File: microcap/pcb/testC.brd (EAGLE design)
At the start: 100 parts

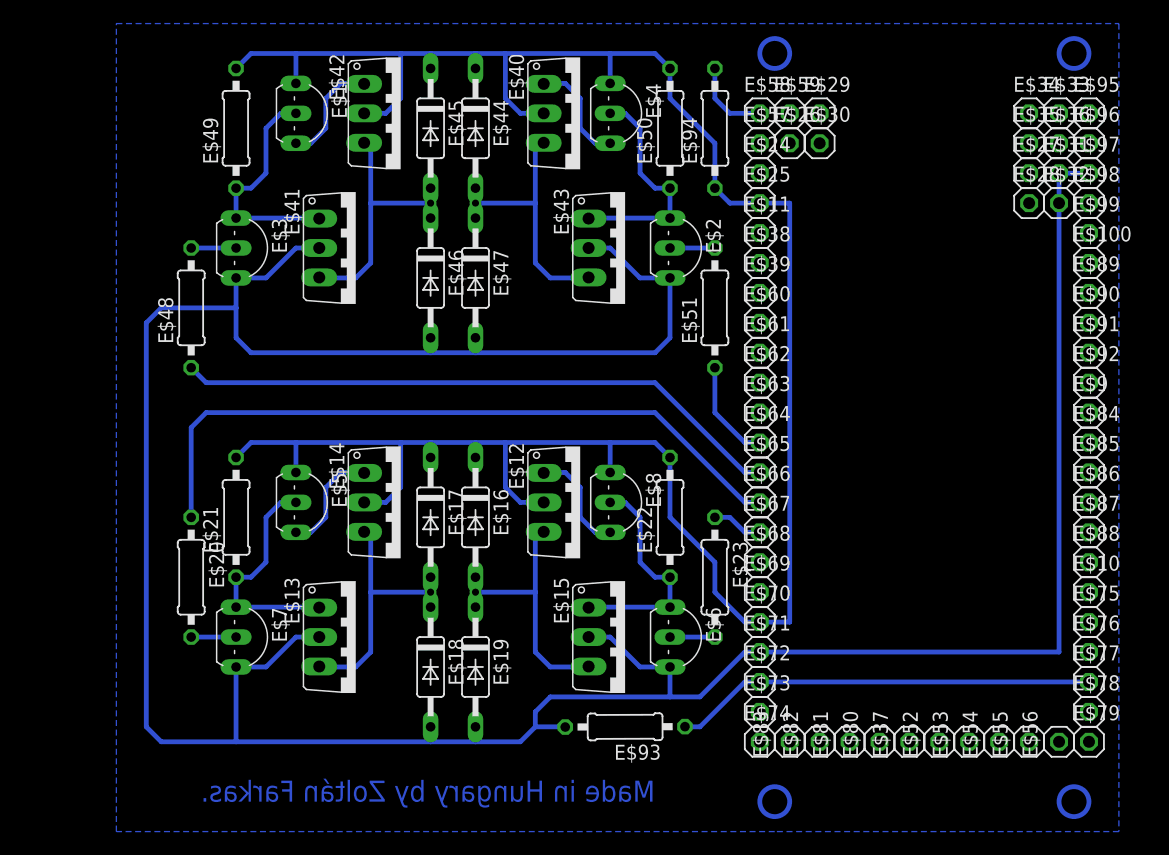
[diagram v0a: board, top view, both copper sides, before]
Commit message: pcb test update
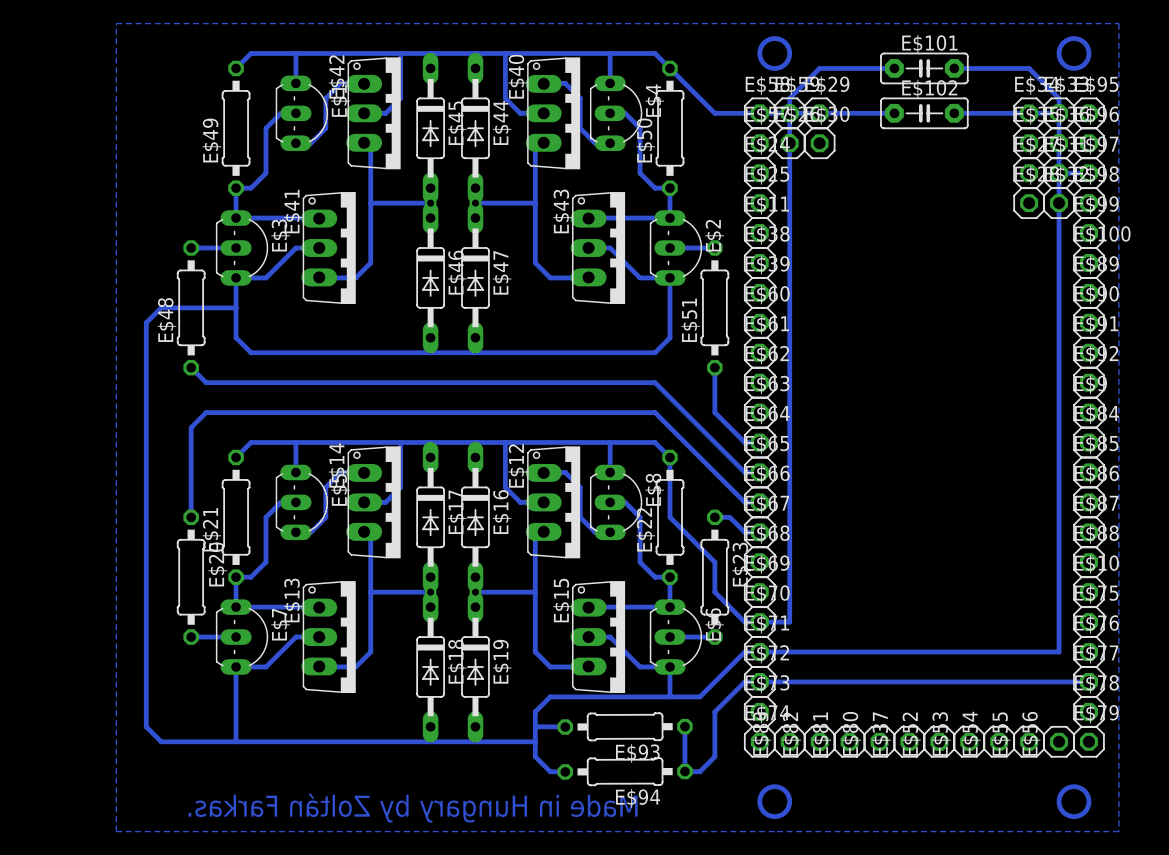
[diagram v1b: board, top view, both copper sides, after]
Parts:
- added E$101, E$102: (no value), capacitor-wima:C5B2.5
- moved E$94 55.1 mm to (71.1, 36.8), turned to 180.2 degrees
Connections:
- removed net S$29: E$1.C, E$16.C, E$17.C, E$21.2, E$22.2, E$25.1, E$4.C, E$44.C, E$45.C, E$49.2, E$5.C, E$50.2, E$70.1, E$8.C, E$94.1
- removed net S$30: E$58.1, E$94.2
- new net S$18: E$101.2, E$102.2, E$18.A, E$19.A, E$2.E, E$3.E, E$46.A, E$47.A, E$6.E, E$7.E, E$71.1, E$97.1
- net S$8: now also E$1.C, E$101.1, E$102.1, E$16.C, E$17.C, E$21.2, E$22.2, E$4.C, E$44.C, E$45.C, E$49.2, E$5.C, E$50.2, E$58.1, E$59.1, E$70.1, E$8.C; no longer E$18.A, E$19.A, E$2.E, E$3.E, E$46.A, E$47.A, E$6.E, E$7.E, E$71.1, E$97.1
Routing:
- net S$18: track 0.00 -> 291.9 mm
- net S$29: track 193.1 -> 0.00 mm
- net S$8: track 261.7 -> 213.9 mm
- net S$26: track 35.9 -> 43.5 mm
- net S$30: track 6.88 -> 0.00 mm
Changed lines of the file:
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@@
 <layer number="21" name="tPlace" color="7" fill="1" visible="yes" active="yes"/>
 <layer number="22" name="bPlace" color="7" fill="1" visible="yes" active="yes"/>
-<layer number="23" name="tOrigins" color="15" fill="1" visible="no" active="yes"/>
-<layer number="24" name="bOrigins" color="15" fill="1" visible="no" active="yes"/>
+<layer number="23" name="tOrigins" color="15" fill="1" visible="yes" active="yes"/>
+<layer number="24" name="bOrigins" color="15" fill="1" visible="yes" active="yes"/>
 <layer number="25" name="tNames" color="7" fill="1" visible="no" active="yes"/>
 <layer number="26" name="bNames" color="7" fill="1" visible="no" active="yes"/>
@@
 <circle x="109.22" y="34.29" radius="1.27" width="0.4064" layer="16"/>
 <circle x="83.82" y="34.29" radius="1.27" width="0.4064" layer="16"/>
-<text x="73.66" y="34.29" size="1.778" layer="16" rot="MR0">Made in Hungary by Zoltán Farkas.</text>
+<text x="72.39" y="33.02" size="1.778" layer="16" rot="MR0">Made in Hungary by Zoltán Farkas.</text>
 </plain>
 <attributes>
@@
 <element name="E$100" library="pinhead" package="1X01" value="" x="110.49" y="80.01"/>
 <element name="E$93" library="resistor" package="0207/10" value="" x="71.12" y="40.64" rot="R180.2"/>
-<element name="E$94" library="resistor" package="0207/10" value="" x="78.74" y="91.44" rot="R90"/>
+<element name="E$94" library="resistor" package="0207/10" value="" x="71.12" y="36.83" rot="R180.2"/>
+<element name="E$101" library="capacitor-wima" package="C5B2.5" value="" x="96.52" y="96.52"/>
+<element name="E$102" library="capacitor-wima" package="C5B2.5" value="" x="96.52" y="92.71"/>
 </elements>
 <signals>
@@
 <wire x1="74.93" y1="81.28" x2="78.74" y2="81.28" width="0.4064" layer="16"/>
 </signal>
-<signal name="S$8">
+<signal name="S$18">
+<wire x1="66.04" y1="36.83" x2="64.77" y2="36.83" width="0.4064" layer="16"/>
 <wire x1="69.85" y1="81.28" x2="68.58" y2="81.28" width="0.4064" layer="16"/>
 <wire x1="72.39" y1="78.74" x2="69.85" y2="81.28" width="0.4064" layer="16"/>
@@
 <wire x1="74.93" y1="45.72" x2="74.93" y2="43.18" width="0.4064" layer="16"/>
 <contactref element="E$18" pad="A"/>
-<wire x1="58.42" y1="39.37" x2="62.23" y2="39.37" width="0.4064" layer="16"/>
+<wire x1="58.42" y1="39.37" x2="63.5" y2="39.37" width="0.4064" layer="16"/>
 <wire x1="58.42" y1="40.64" x2="58.42" y2="39.37" width="0.4064" layer="16"/>
 <contactref element="E$7" pad="E"/>
@@
 <wire x1="63.5" y1="41.91" x2="63.5" y2="40.64" width="0.4064" layer="16"/>
 <wire x1="66.04" y1="40.64" x2="63.5" y2="40.64" width="0.4064" layer="16"/>
-<wire x1="63.5" y1="40.64" x2="62.23" y2="39.37" width="0.4064" layer="16"/>
+<wire x1="63.5" y1="38.1" x2="63.5" y2="39.37" width="0.4064" layer="16"/>
+<wire x1="63.5" y1="39.37" x2="63.5" y2="40.64" width="0.4064" layer="16"/>
+<wire x1="64.77" y1="36.83" x2="63.5" y2="38.1" width="0.4064" layer="16"/>
+<wire x1="107.95" y1="87.63" x2="107.95" y2="92.71" width="0.4064" layer="16"/>
+<contactref element="E$101" pad="2"/>
+<wire x1="107.95" y1="92.71" x2="107.95" y2="93.98" width="0.4064" layer="16"/>
+<wire x1="99.06" y1="96.52" x2="105.41" y2="96.52" width="0.4064" layer="16"/>
+<wire x1="105.41" y1="96.52" x2="107.95" y2="93.98" width="0.4064" layer="16"/>
+<contactref element="E$102" pad="2"/>
+<wire x1="99.06" y1="92.71" x2="107.95" y2="92.71" width="0.4064" layer="16"/>
 </signal>
 <signal name="S$1">
@@
 </signal>
 <signal name="S$26">
+<wire x1="76.2" y1="36.83" x2="77.47" y2="36.83" width="0.4064" layer="16"/>
+<wire x1="77.47" y1="36.83" x2="78.74" y2="38.1" width="0.4064" layer="16"/>
 <contactref element="E$77" pad="1"/>
 <wire x1="110.49" y1="44.45" x2="81.28" y2="44.45" width="0.4064" layer="16"/>
-<wire x1="81.28" y1="44.45" x2="77.47" y2="40.64" width="0.4064" layer="16"/>
-<wire x1="77.47" y1="40.64" x2="76.2" y2="40.64" width="0.4064" layer="16"/>
-</signal>
-<signal name="S$30">
-<contactref element="E$94" pad="2"/>
-<wire x1="78.74" y1="93.98" x2="78.74" y2="96.52" width="0.4064" layer="16"/>
-<contactref element="E$58" pad="1"/>
-<wire x1="82.55" y1="92.71" x2="80.01" y2="92.71" width="0.4064" layer="16"/>
-<wire x1="80.01" y1="92.71" x2="78.74" y2="93.98" width="0.4064" layer="16"/>
-</signal>
-<signal name="S$29">
-<contactref element="E$25" pad="1"/>
-<contactref element="E$50" pad="2"/>
-<contactref element="E$4" pad="C"/>
-<wire x1="73.66" y1="97.79" x2="74.93" y2="96.52" width="0.4064" layer="16"/>
-<wire x1="63.5" y1="92.71" x2="62.23" y2="92.71" width="0.4064" layer="16"/>
-<wire x1="62.23" y1="92.71" x2="60.96" y2="93.98" width="0.4064" layer="16"/>
-<wire x1="69.85" y1="97.79" x2="73.66" y2="97.79" width="0.4064" layer="16"/>
-<wire x1="69.85" y1="95.25" x2="69.85" y2="97.79" width="0.4064" layer="16"/>
-<contactref element="E$44" pad="C"/>
-<wire x1="60.96" y1="97.79" x2="69.85" y2="97.79" width="0.4064" layer="16"/>
-<wire x1="60.96" y1="93.98" x2="60.96" y2="97.79" width="0.4064" layer="16"/>
-<contactref element="E$45" pad="C"/>
-<wire x1="58.42" y1="97.79" x2="60.96" y2="97.79" width="0.4064" layer="16"/>
-<wire x1="58.42" y1="96.52" x2="58.42" y2="97.79" width="0.4064" layer="16"/>
-<wire x1="49.53" y1="92.71" x2="50.8" y2="92.71" width="0.4064" layer="16"/>
-<wire x1="50.8" y1="92.71" x2="52.07" y2="93.98" width="0.4064" layer="16"/>
-<wire x1="54.61" y1="97.79" x2="58.42" y2="97.79" width="0.4064" layer="16"/>
-<wire x1="54.61" y1="96.52" x2="54.61" y2="97.79" width="0.4064" layer="16"/>
-<contactref element="E$1" pad="C"/>
-<wire x1="52.07" y1="97.79" x2="54.61" y2="97.79" width="0.4064" layer="16"/>
-<wire x1="52.07" y1="93.98" x2="52.07" y2="97.79" width="0.4064" layer="16"/>
-<contactref element="E$49" pad="2"/>
-<wire x1="43.18" y1="97.79" x2="52.07" y2="97.79" width="0.4064" layer="16"/>
-<wire x1="43.18" y1="95.25" x2="43.18" y2="97.79" width="0.4064" layer="16"/>
-<wire x1="39.37" y1="97.79" x2="43.18" y2="97.79" width="0.4064" layer="16"/>
-<wire x1="38.1" y1="96.52" x2="39.37" y2="97.79" width="0.4064" layer="16"/>
-<wire x1="74.93" y1="96.52" x2="74.93" y2="93.98" width="0.4064" layer="16"/>
-<wire x1="74.93" y1="93.98" x2="78.74" y2="90.17" width="0.4064" layer="16"/>
-<contactref element="E$94" pad="1"/>
-<wire x1="78.74" y1="90.17" x2="78.74" y2="86.36" width="0.4064" layer="16"/>
-<wire x1="82.55" y1="85.09" x2="80.01" y2="85.09" width="0.4064" layer="16"/>
-<wire x1="80.01" y1="85.09" x2="78.74" y2="86.36" width="0.4064" layer="16"/>
+<wire x1="81.28" y1="44.45" x2="78.74" y2="41.91" width="0.4064" layer="16"/>
+<wire x1="78.74" y1="38.1" x2="78.74" y2="41.91" width="0.4064" layer="16"/>
+<wire x1="76.2" y1="36.83" x2="76.2" y2="40.64" width="0.4064" layer="16"/>
+</signal>
+<signal name="S$8">
+<contactref element="E$101" pad="1"/>
 <contactref element="E$70" pad="1"/>
-<wire x1="85.09" y1="85.09" x2="85.09" y2="49.53" width="0.4064" layer="16"/>
+<wire x1="85.09" y1="92.71" x2="85.09" y2="49.53" width="0.4064" layer="16"/>
 <wire x1="82.55" y1="49.53" x2="81.28" y2="49.53" width="0.4064" layer="16"/>
 <wire x1="85.09" y1="49.53" x2="82.55" y2="49.53" width="0.4064" layer="16"/>
@@
 <wire x1="78.74" y1="54.61" x2="78.74" y2="52.07" width="0.4064" layer="16"/>
 <wire x1="81.28" y1="49.53" x2="78.74" y2="52.07" width="0.4064" layer="16"/>
-<wire x1="82.55" y1="85.09" x2="85.09" y2="85.09" width="0.4064" layer="16"/>
+<contactref element="E$59" pad="1"/>
+<contactref element="E$58" pad="1"/>
+<wire x1="85.09" y1="92.71" x2="82.55" y2="92.71" width="0.4064" layer="16"/>
+<contactref element="E$50" pad="2"/>
+<contactref element="E$4" pad="C"/>
+<wire x1="73.66" y1="97.79" x2="74.93" y2="96.52" width="0.4064" layer="16"/>
+<wire x1="63.5" y1="92.71" x2="62.23" y2="92.71" width="0.4064" layer="16"/>
+<wire x1="62.23" y1="92.71" x2="60.96" y2="93.98" width="0.4064" layer="16"/>
+<wire x1="69.85" y1="97.79" x2="73.66" y2="97.79" width="0.4064" layer="16"/>
+<wire x1="69.85" y1="95.25" x2="69.85" y2="97.79" width="0.4064" layer="16"/>
+<contactref element="E$44" pad="C"/>
+<wire x1="60.96" y1="97.79" x2="69.85" y2="97.79" width="0.4064" layer="16"/>
+<wire x1="60.96" y1="93.98" x2="60.96" y2="97.79" width="0.4064" layer="16"/>
+<contactref element="E$45" pad="C"/>
+<wire x1="58.42" y1="97.79" x2="60.96" y2="97.79" width="0.4064" layer="16"/>
+<wire x1="58.42" y1="96.52" x2="58.42" y2="97.79" width="0.4064" layer="16"/>
+<wire x1="49.53" y1="92.71" x2="50.8" y2="92.71" width="0.4064" layer="16"/>
+<wire x1="50.8" y1="92.71" x2="52.07" y2="93.98" width="0.4064" layer="16"/>
+<wire x1="54.61" y1="97.79" x2="58.42" y2="97.79" width="0.4064" layer="16"/>
+<wire x1="54.61" y1="96.52" x2="54.61" y2="97.79" width="0.4064" layer="16"/>
+<contactref element="E$1" pad="C"/>
+<wire x1="52.07" y1="97.79" x2="54.61" y2="97.79" width="0.4064" layer="16"/>
+<wire x1="52.07" y1="93.98" x2="52.07" y2="97.79" width="0.4064" layer="16"/>
+<contactref element="E$49" pad="2"/>
+<wire x1="43.18" y1="97.79" x2="52.07" y2="97.79" width="0.4064" layer="16"/>
+<wire x1="43.18" y1="95.25" x2="43.18" y2="97.79" width="0.4064" layer="16"/>
+<wire x1="39.37" y1="97.79" x2="43.18" y2="97.79" width="0.4064" layer="16"/>
+<wire x1="38.1" y1="96.52" x2="39.37" y2="97.79" width="0.4064" layer="16"/>
+<wire x1="82.55" y1="92.71" x2="78.74" y2="92.71" width="0.4064" layer="16"/>
+<wire x1="78.74" y1="92.71" x2="74.93" y2="96.52" width="0.4064" layer="16"/>
+<wire x1="85.09" y1="92.71" x2="85.09" y2="93.98" width="0.4064" layer="16"/>
+<wire x1="93.98" y1="96.52" x2="87.63" y2="96.52" width="0.4064" layer="16"/>
+<wire x1="87.63" y1="96.52" x2="85.09" y2="93.98" width="0.4064" layer="16"/>
+<contactref element="E$102" pad="1"/>
+<wire x1="85.09" y1="92.71" x2="93.98" y2="92.71" width="0.4064" layer="16"/>
 </signal>
 </signals>
